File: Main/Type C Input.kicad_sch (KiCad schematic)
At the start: 12 parts, among them J1 12402012E212A, U1 STUSB4500LQTR, U2 ESDA25L

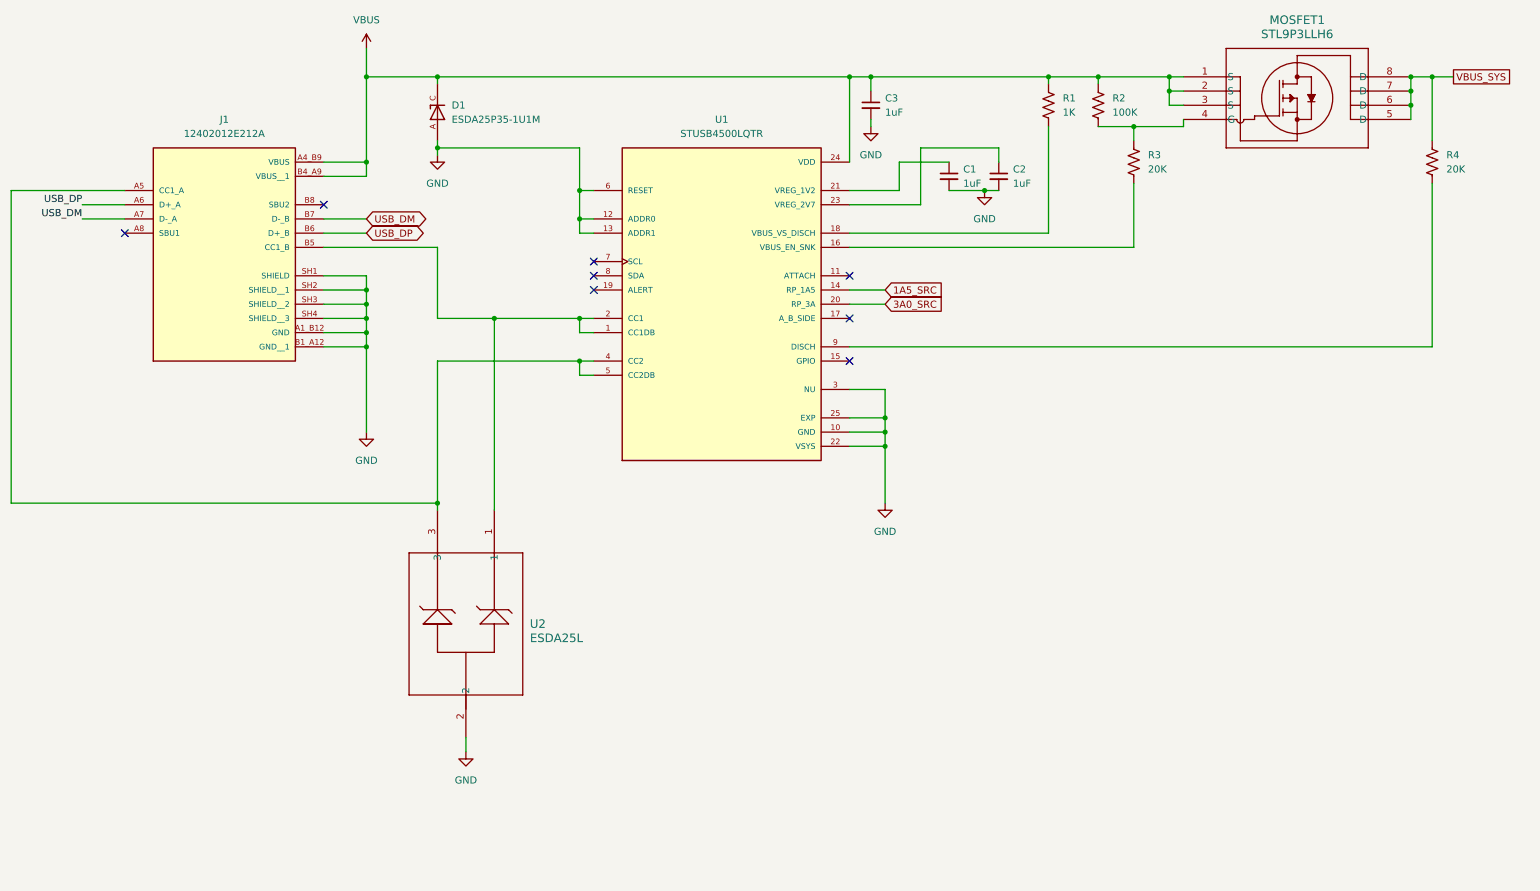
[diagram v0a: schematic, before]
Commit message: Add files via upload
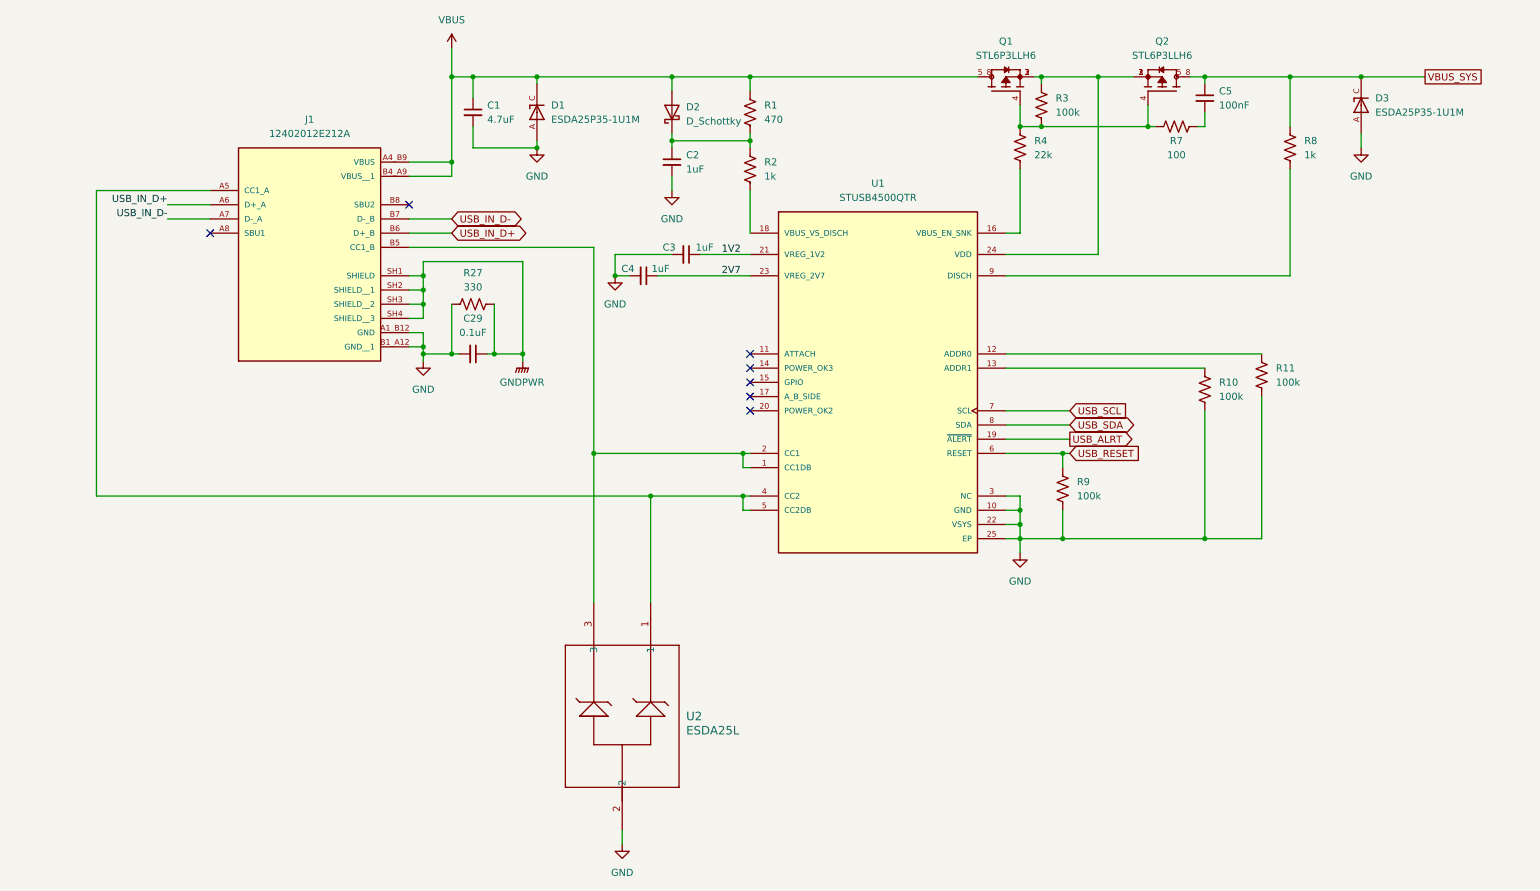
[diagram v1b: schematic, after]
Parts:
- removed MOSFET1: STL9P3LLH6, POWERFLAT_3P3X3P3_STM, symbol STL9P3LLH6:STL9P3LLH6
- removed U1: STUSB4500LQTR, STUSB4500LQTR:QFN50P400X400X100-25N, symbol STUSB4500LQTR:STUSB4500LQTR
- added C29: 0.1uF, symbol Device:C_Small
- added C4: 1uF, symbol Device:C_Small
- added C5: 100nF, symbol Device:C_Small
- added D2: D_Schottky, symbol Device:D_Schottky
- added D3: ESDA25P35-1U1M, ESDA25P35-1U1M:TVS_ESDA25P35-1U1M, symbol ESDA25P35:ESDA25P35-1U1M
- added Q1, Q2: STL6P3LLH6, STL6P3LLH6:TRANS_STL6P3LLH6, symbol STL6P3LLH6:STL6P3LLH6
- added R10, R11, R9: 100k, symbol Device:R_US
- added R27: 330, symbol Device:R_US
- added R7: 100, symbol Device:R_US
- added R8: 1k, symbol Device:R_US
- added U1: STUSB4500QTR, STUSB4500QTR:QFN50P400X400X90-25N, symbol STUSB4500QTR:STUSB4500QTR
- C1: value 1uF -> 4.7uF; footprint Capacitor_SMD:C_0805_2012Metric_Pad1.18x1.45mm_HandSolder -> (none)
- C2, C3: footprint Capacitor_SMD:C_0805_2012Metric_Pad1.18x1.45mm_HandSolder -> (none)
- R1: value 1K -> 470
- R2: value 100K -> 1k
- R3: value 20K -> 100k
- R4: value 20K -> 22k
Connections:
- net GND: now also C29.2, C4.2, D3.A, R10.2, R11.2, R27.1, R9.2, U1.10 (GND), U1.22 (VSYS), U1.25 (EP), U1.3 (NC); no longer J1.SH1 (SHIELD), J1.SH2 (SHIELD__1), J1.SH3 (SHIELD__2), J1.SH4 (SHIELD__3)
- net VBUS: now also C1.1, D2.2 (A), Q1.5_8; no longer C3.1, R2.1
- net VBUS_SYS: now also C5.1, D3.C, Q2.5_8, R8.1; no longer R4.1
- net at U2.1: now also J1.A5 (CC1_A), U1.4 (CC2), U1.5 (CC2DB); no longer J1.B5 (CC1_B)
- net at U2.3: now also J1.B5 (CC1_B), U1.1 (CC1DB), U1.2 (CC1); no longer J1.A5 (CC1_A)
- net at C2.1: now also R1.2, R2.1, D2.1 (K)
- net at R3.2: now also R4.1, Q1.4, Q2.4, R7.2
- net at R4.2: now also U1.16 (VBUS_EN_SNK)
- net at R2.2: now also U1.18 (VBUS_VS_DISCH); no longer R3.1
- net USB_DM renamed USB_IN_D-
- net USB_DP renamed USB_IN_D+
- new net: R10.1, U1.13 (ADDR1)
- new net: Q1.1, Q1.2, Q1.3, Q2.1, Q2.2, Q2.3, R3.1, U1.24 (VDD)
- new net: C5.2, R7.1
- new net: R8.2, U1.9 (DISCH)
- new net: R11.1, U1.12 (ADDR0)
- new net 1V2: C3.1, U1.21 (VREG_1V2)
- new net 2V7: C4.1, U1.23 (VREG_2V7)
- new net GNDPWR: C29.1, J1.SH1 (SHIELD), J1.SH2 (SHIELD__1), J1.SH3 (SHIELD__2), J1.SH4 (SHIELD__3), R27.2
- new net USB_ALRT: U1.19 (~{ALERT})
- new net USB_RESET: R9.1, U1.6 (RESET)
- new net USB_SCL: U1.7 (SCL)
- new net USB_SDA: U1.8 (SDA)
- no-connect marks 8 -> 7
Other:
- moved on the sheet: J1, U2
